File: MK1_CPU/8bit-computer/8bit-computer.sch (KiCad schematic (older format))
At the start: 16 parts, among them J1 USB_B-8bit-computer-rescue, J2 Barrel_Jack_Switch, U1 74HCT32, U2 74HCT32

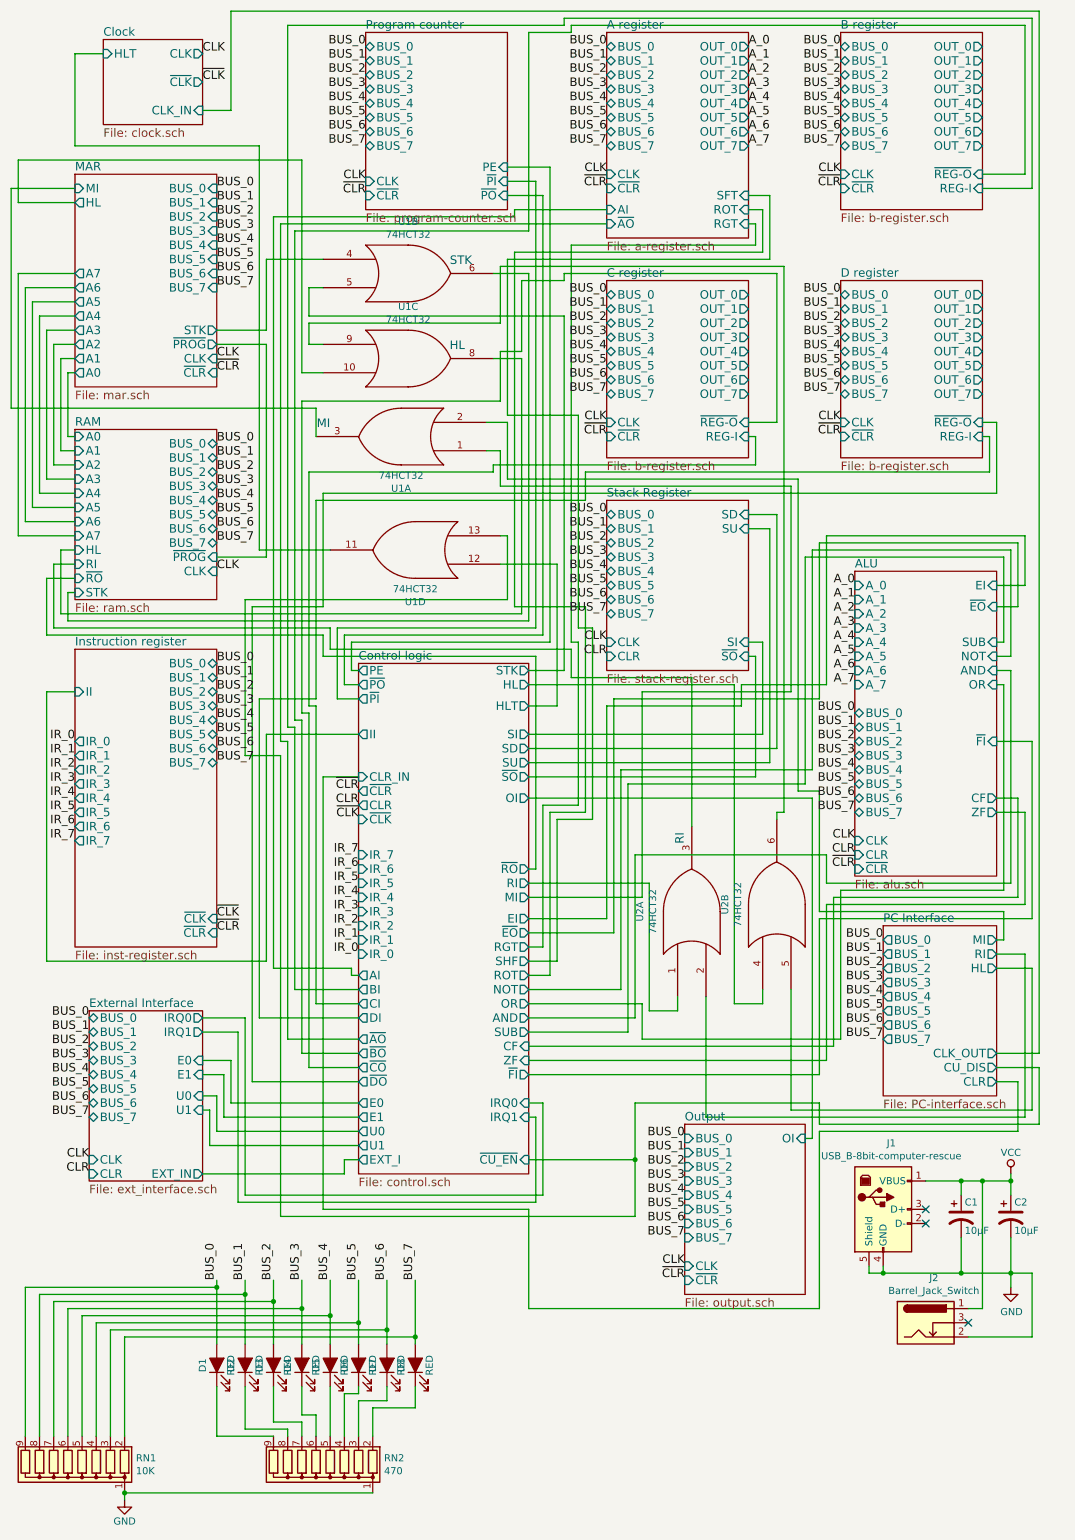
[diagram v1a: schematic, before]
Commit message: schematics cleanup
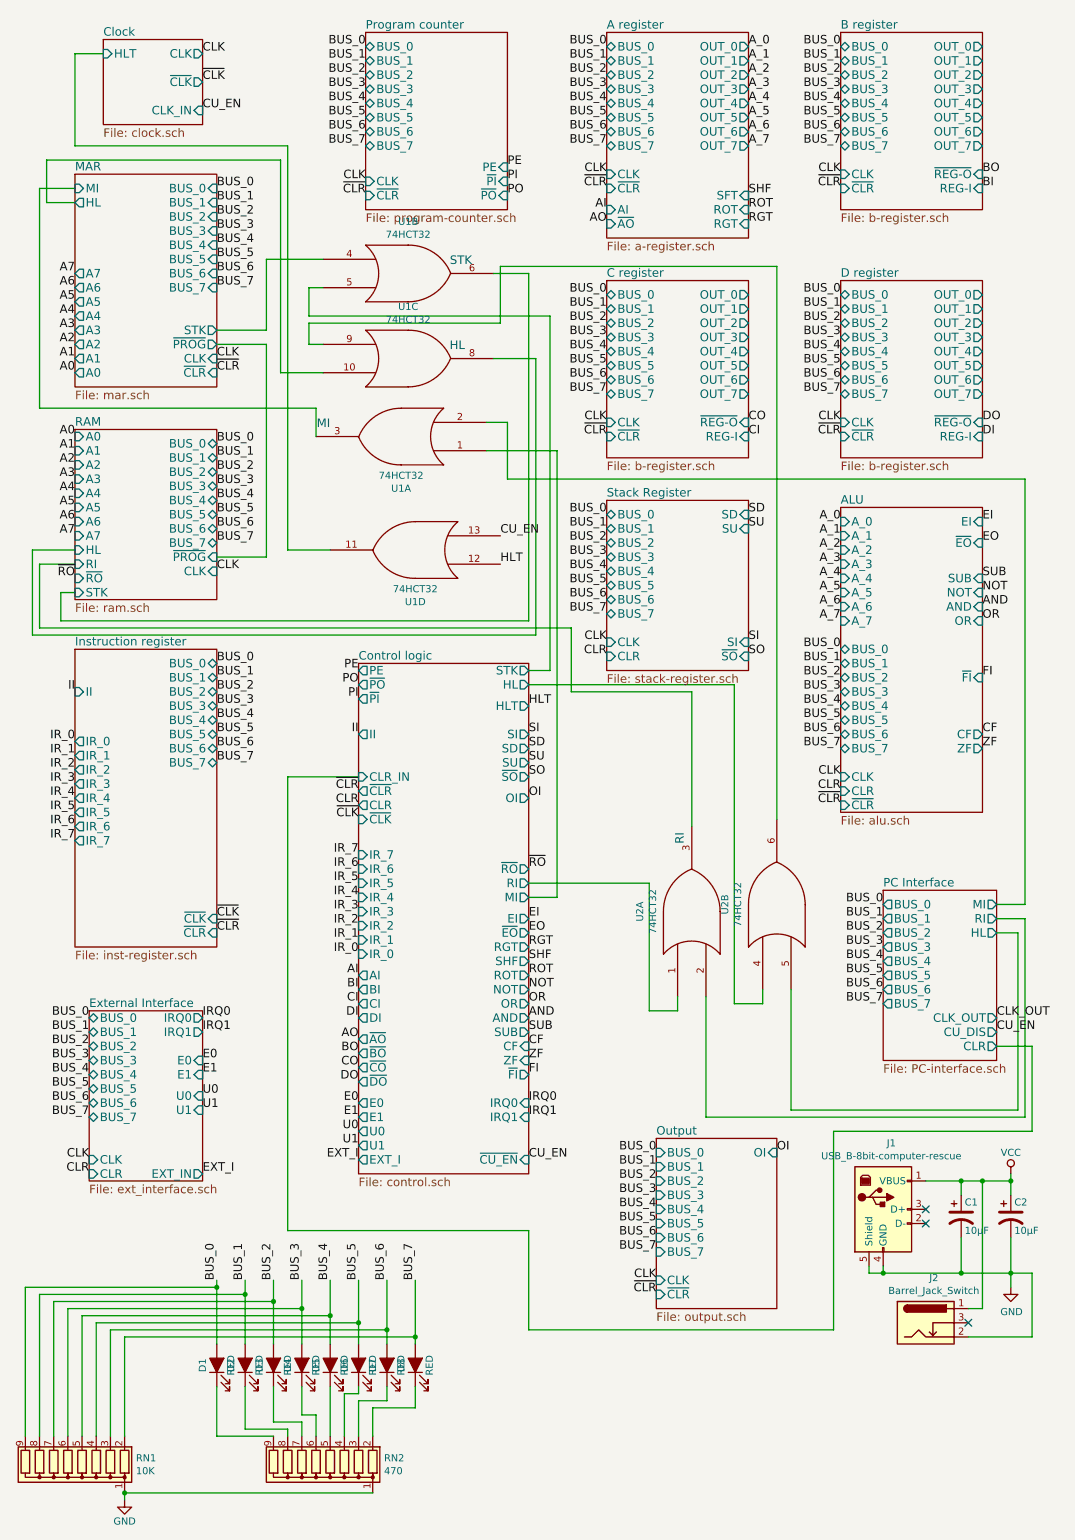
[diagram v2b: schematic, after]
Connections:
- net Control logic/HLT renamed HLT
- net Control logic/~CU_EN renamed CU_EN
